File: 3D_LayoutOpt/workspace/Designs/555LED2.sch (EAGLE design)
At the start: 10 parts, among them IC1 555, IC2 555, IC3 555, IC4 555

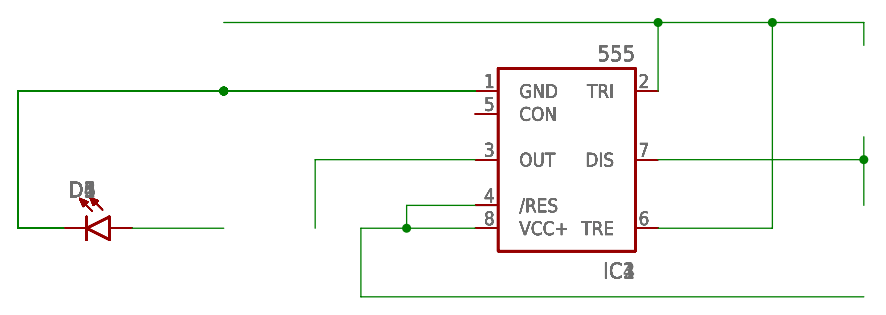
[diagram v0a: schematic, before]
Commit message: Code works!
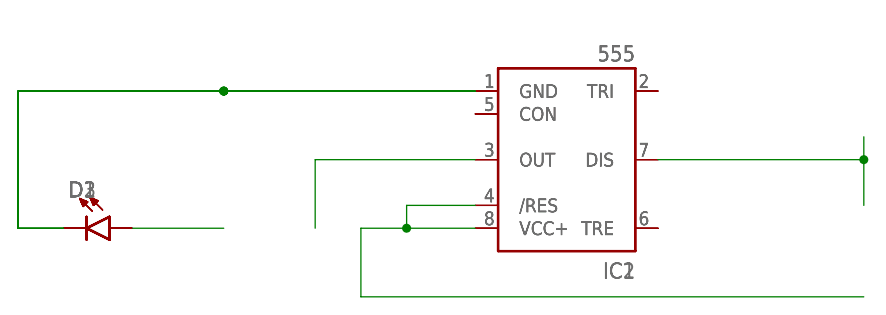
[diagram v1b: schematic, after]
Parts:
- removed D4, D5, D6: (no value), SparkFun-LED:LED1206
- removed IC3, IC4: 555, SparkFun-IC-Special-Function:555D
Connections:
- removed net N$7: D1.C, D4.A, IC2.DIS
- removed net N$8: D3.A, D6.C, IC1.GND, IC2.OUT, IC3.DIS
- net N$3: now also D3.A, IC2.VCC+; no longer D4.A, IC4.VCC+
- net N$4: now also D3.A, IC2.DIS; no longer D5.A, IC3.GND
- net N$5: now also D2.C, D3.A, IC2.GND; no longer D5.A, D6.C, IC1.TRI, IC3.TRE
- net N$6: now also D3.A, IC1.GND, IC2.OUT; no longer D4.A, IC2.GND
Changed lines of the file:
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@@
 <part name="IC1" library="SparkFun-IC-Special-Function" deviceset="555" device="D" value="555"/>
 <part name="IC2" library="SparkFun-IC-Special-Function" deviceset="555" device="D" value="555"/>
-<part name="IC3" library="SparkFun-IC-Special-Function" deviceset="555" device="D" value="555"/>
-<part name="IC4" library="SparkFun-IC-Special-Function" deviceset="555" device="D" value="555"/>
 <part name="D1" library="SparkFun-LED" deviceset="LED" device="1206"/>
 <part name="D2" library="SparkFun-LED" deviceset="LED" device="1206"/>
 <part name="D3" library="SparkFun-LED" deviceset="LED" device="1206"/>
-<part name="D4" library="SparkFun-LED" deviceset="LED" device="1206"/>
-<part name="D5" library="SparkFun-LED" deviceset="LED" device="1206"/>
-<part name="D6" library="SparkFun-LED" deviceset="LED" device="1206"/>
 </parts>
 <sheets>
@@
 <instance part="IC1" gate="G$1" x="50.8" y="58.42" rot="R180"/>
 <instance part="IC2" gate="G$1" x="50.8" y="58.42" rot="R180"/>
-<instance part="IC3" gate="G$1" x="50.8" y="58.42" rot="R180"/>
-<instance part="IC4" gate="G$1" x="50.8" y="58.42" rot="R180"/>
 <instance part="D1" gate="G$1" x="0" y="50.8" rot="R270"/>
 <instance part="D2" gate="G$1" x="0" y="50.8" rot="R270"/>
 <instance part="D3" gate="G$1" x="0" y="50.8" rot="R270"/>
-<instance part="D4" gate="G$1" x="0" y="50.8" rot="R270"/>
-<instance part="D5" gate="G$1" x="0" y="50.8" rot="R270"/>
-<instance part="D6" gate="G$1" x="0" y="50.8" rot="R270"/>
 </instances>
 <busses>
@@
 <wire x1="40.64" y1="53.34" x2="33.02" y2="53.34" width="0.1524" layer="91"/>
 <wire x1="33.02" y1="53.34" x2="33.02" y2="50.8" width="0.1524" layer="91"/>
-<pinref part="IC4" gate="G$1" pin="VCC+"/>
+<pinref part="IC2" gate="G$1" pin="VCC+"/>
 <wire x1="33.02" y1="50.8" x2="40.64" y2="50.8" width="0.1524" layer="91"/>
-<pinref part="D4" gate="G$1" pin="A"/>
+<pinref part="D3" gate="G$1" pin="A"/>
 <wire x1="83.82" y1="43.18" x2="27.94" y2="43.18" width="0.1524" layer="91"/>
 <wire x1="27.94" y1="43.18" x2="27.94" y2="50.8" width="0.1524" layer="91"/>
@@
 </segment>
 </net>
-<net name="N$5" class="0">
-<segment>
-<pinref part="IC1" gate="G$1" pin="TRI"/>
-<wire x1="60.96" y1="73.66" x2="60.96" y2="66.04" width="0.1524" layer="91"/>
-<pinref part="D5" gate="G$1" pin="A"/>
-<wire x1="60.96" y1="73.66" x2="73.66" y2="73.66" width="0.1524" layer="91"/>
-<wire x1="73.66" y1="73.66" x2="83.82" y2="73.66" width="0.1524" layer="91"/>
-<wire x1="83.82" y1="73.66" x2="83.82" y2="71.12" width="0.1524" layer="91"/>
-<pinref part="IC3" gate="G$1" pin="TRE"/>
-<wire x1="60.96" y1="50.8" x2="73.66" y2="50.8" width="0.1524" layer="91"/>
-<wire x1="73.66" y1="50.8" x2="73.66" y2="73.66" width="0.1524" layer="91"/>
-<junction x="73.66" y="73.66"/>
-<pinref part="D6" gate="G$1" pin="C"/>
-<wire x1="12.7" y1="73.66" x2="60.96" y2="73.66" width="0.1524" layer="91"/>
-<junction x="60.96" y="73.66"/>
-</segment>
-</net>
-<net name="N$7" class="0">
+<net name="N$4" class="0">
 <segment>
 <pinref part="D1" gate="G$1" pin="C"/>
-<pinref part="D4" gate="G$1" pin="A"/>
+<pinref part="D3" gate="G$1" pin="A"/>
 <wire x1="83.82" y1="60.96" x2="83.82" y2="58.42" width="0.1524" layer="91"/>
 <pinref part="IC2" gate="G$1" pin="DIS"/>
@@
 </segment>
 </net>
-<net name="N$4" class="0">
+<net name="N$5" class="0">
 <segment>
-<pinref part="D1" gate="G$1" pin="C"/>
+<pinref part="D2" gate="G$1" pin="C"/>
 <wire x1="-5.08" y1="50.8" x2="-10.16" y2="50.8" width="0.1524" layer="91"/>
 <wire x1="-10.16" y1="50.8" x2="-10.16" y2="66.04" width="0.1524" layer="91"/>
-<pinref part="D5" gate="G$1" pin="A"/>
+<pinref part="D3" gate="G$1" pin="A"/>
 <wire x1="-10.16" y1="66.04" x2="12.7" y2="66.04" width="0.1524" layer="91"/>
-<pinref part="IC3" gate="G$1" pin="GND"/>
+<pinref part="IC2" gate="G$1" pin="GND"/>
 <wire x1="12.7" y1="66.04" x2="40.64" y2="66.04" width="0.1524" layer="91"/>
 <junction x="12.7" y="66.04"/>
@@
 <wire x1="-5.08" y1="50.8" x2="-10.16" y2="50.8" width="0.1524" layer="91"/>
 <wire x1="-10.16" y1="50.8" x2="-10.16" y2="66.04" width="0.1524" layer="91"/>
-<pinref part="D4" gate="G$1" pin="A"/>
-<wire x1="-10.16" y1="66.04" x2="12.7" y2="66.04" width="0.1524" layer="91"/>
-<pinref part="IC2" gate="G$1" pin="GND"/>
-<wire x1="12.7" y1="66.04" x2="40.64" y2="66.04" width="0.1524" layer="91"/>
-<junction x="12.7" y="66.04"/>
-</segment>
-</net>
-<net name="N$8" class="0">
-<segment>
-<pinref part="D6" gate="G$1" pin="C"/>
-<wire x1="-5.08" y1="50.8" x2="-10.16" y2="50.8" width="0.1524" layer="91"/>
-<wire x1="-10.16" y1="50.8" x2="-10.16" y2="66.04" width="0.1524" layer="91"/>
 <pinref part="D3" gate="G$1" pin="A"/>
 <wire x1="-10.16" y1="66.04" x2="12.7" y2="66.04" width="0.1524" layer="91"/>
 <pinref part="IC1" gate="G$1" pin="GND"/>
 <pinref part="IC2" gate="G$1" pin="OUT"/>
-<pinref part="IC3" gate="G$1" pin="DIS"/>
 <wire x1="12.7" y1="66.04" x2="40.64" y2="66.04" width="0.1524" layer="91"/>
 <junction x="12.7" y="66.04"/>
